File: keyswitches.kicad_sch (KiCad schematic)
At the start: 79 parts, among them U10 KEY_LARR, U11 KEY_STOP, U12 KEY_SPACE, U13 KEY_Q, U14 KEY_1, U15 KEY_SHIFTLOCK, U16 KEY_LSHIFT, U17 KEY_ESC, U18 KEY_>, U19 KEY_A, U20 KEY_W, U21 KEY_2, U22 KEY_Z, U23 KEY_ALT, U24 KEY_0, U25 KEY_P, U26 KEY_:, U27 KEY_?, U28 KEY_LEFT, U29 KEY_E, U30 KEY_S, U31 KEY_3, U32 KEY_X, U33 KEY_@, U34 KEY_+, U35 KEY_;, U36 KEY_CAPSLOCK, U37 KEY_R, U38 KEY_D, U39 KEY_4, U40 KEY_C, U41 KEY_DOWN, U42 KEY_RSHIFT, U43 KEY_*, U44 KEY_-, U45 KEY_=, U46 KEY_T, U47 KEY_F, U48 KEY_5, U49 KEY_V, U50 KEY_NOSCRL, U51 KEY_UP, U52 KEY_RIGHT, U53 KEY_GBP, U54 KEY_Y, U55 KEY_G, U56 KEY_6, U57 KEY_UPARW, U58 KEY_B, U59 KEY_F1, U60 KEY_F9, U61 KEY_HOME, U62 KEY_RETURN, U63 KEY_U, U64 KEY_H, U65 KEY_7, U66 KEY_N, U67 KEY_RESTORE, U68 KEY_F3, U69 KEY_F11, U7 KEY_MEGA, U70 KEY_DEL, U71 KEY_I, U72 KEY_J, U73 KEY_8, U74 KEY_M, U75 KEY_F5, U76 KEY_F13, U77 KEY_O, U78 KEY_K, U79 KEY_9, U8 KEY_TAB, U80 KEY_<, U81 KEY_F7, U82 KEY_HELP, U83 KEY_L, U9 KEY_CTRL

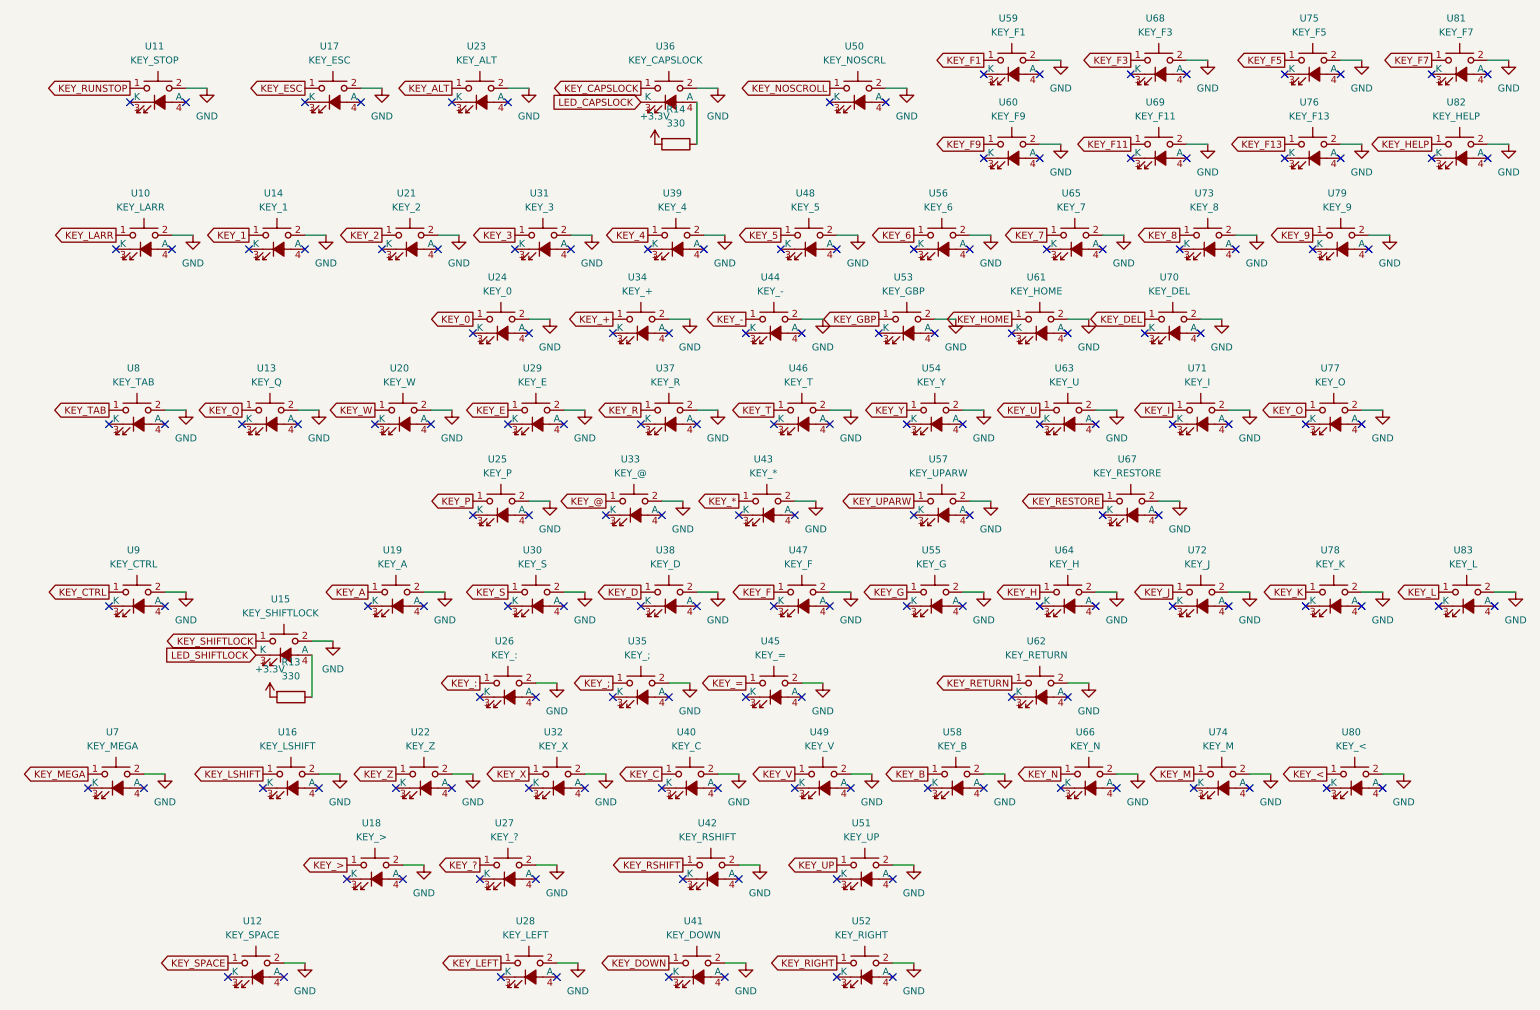
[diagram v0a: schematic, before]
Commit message: tweak PCB appearance
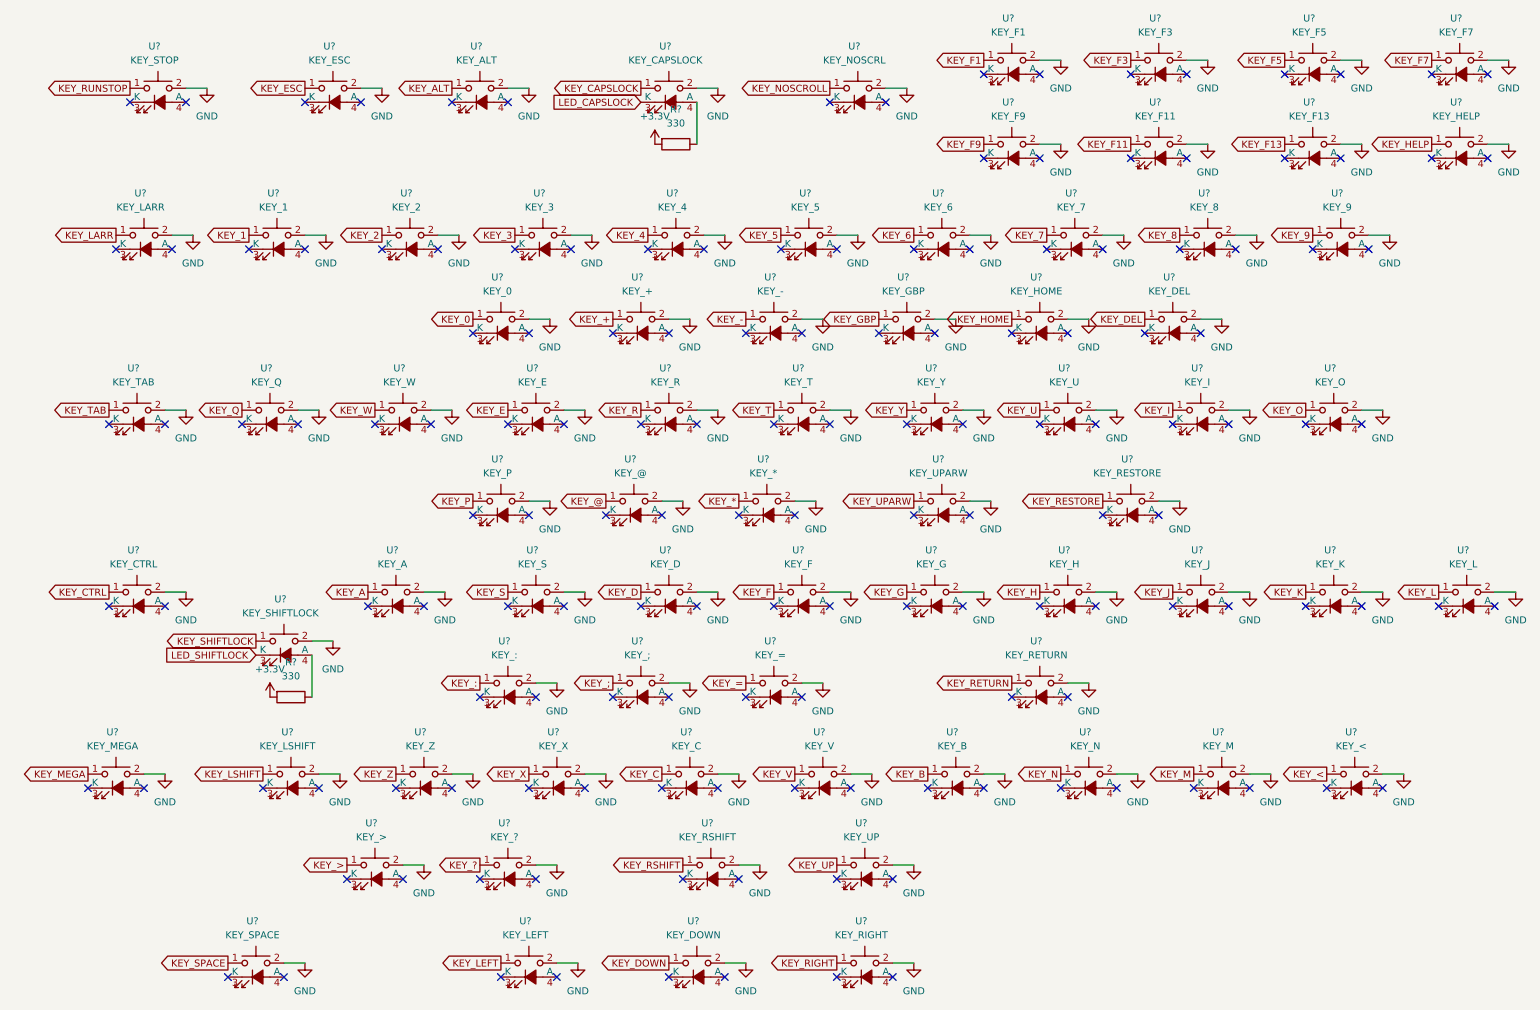
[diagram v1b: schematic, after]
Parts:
- renumbered R13 to R?, R14 to R?, U19 to U?, U68 to U?, U67 to U?, U78 to U?, U66 to U?, U75 to U?, U29 to U?, U14 to U?, U21 to U?, U49 to U?, U32 to U?, U47 to U?, U55 to U?, U65 to U?, U53 to U?, U60 to U?, U38 to U?, U69 to U?, U74 to U?, U70 to U?, U54 to U?, U37 to U?, U8 to U?, U16 to U?, U46 to U?, U23 to U?, U30 to U?, U25 to U?, U13 to U?, U24 to U?, U36 to U?, U72 to U?, U12 to U?, U34 to U?, U79 to U?, U26 to U?, U43 to U?, U51 to U?, U57 to U?, U83 to U?, U41 to U?, U18 to U?, U76 to U?, U52 to U?, U39 to U?, U9 to U?, U77 to U?, U73 to U?, U61 to U?, U20 to U?, U59 to U?, U42 to U?, U62 to U?, U81 to U?, U80 to U?, U15 to U?, U22 to U?, U48 to U?, U63 to U?, U50 to U?, U64 to U?, U35 to U?, U45 to U?, U7 to U?, U17 to U?, U82 to U?, U71 to U?, U44 to U?, U27 to U?, U11 to U?, U10 to U?, U31 to U?, U33 to U?, U40 to U?, U28 to U?, U56 to U?, U58 to U?

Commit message: improve keyswitch footprint to show key IDs
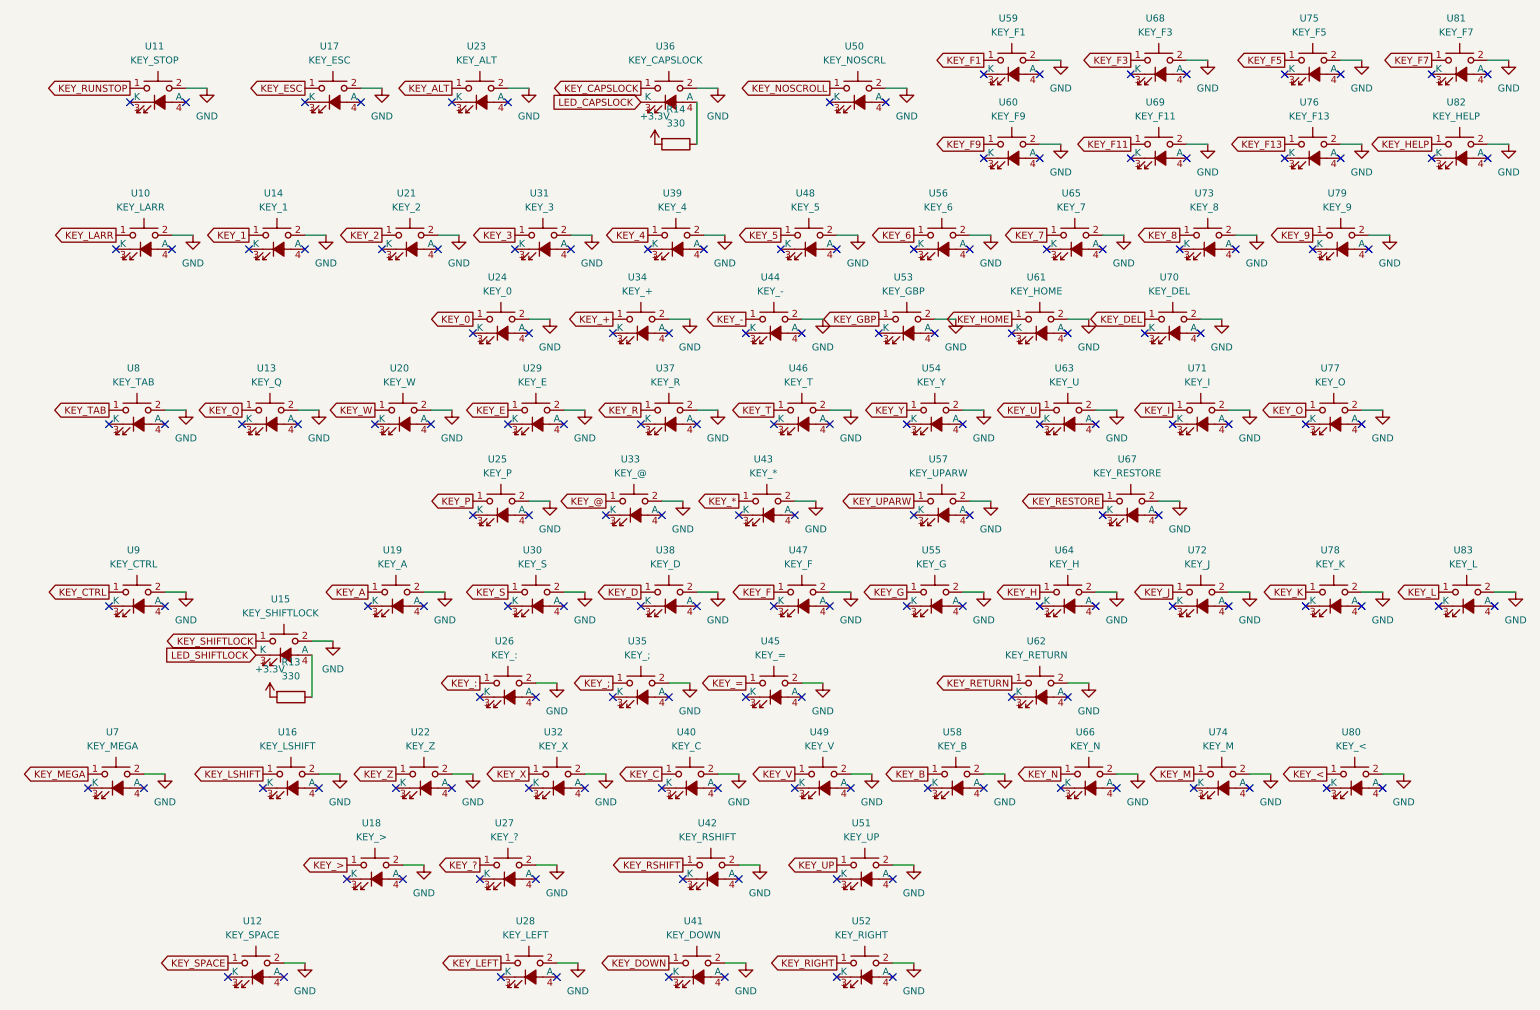
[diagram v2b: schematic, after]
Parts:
- gave numbers to parts that had none: 79
